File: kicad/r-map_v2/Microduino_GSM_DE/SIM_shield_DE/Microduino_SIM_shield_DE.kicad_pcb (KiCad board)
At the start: 2 copper layers, 25.5 x 27.9 mm, 15 parts, among them P1 CONN_1x27, P2 CONN_01X06, U1 TLV62569, U2 ESDA6V1-5W6

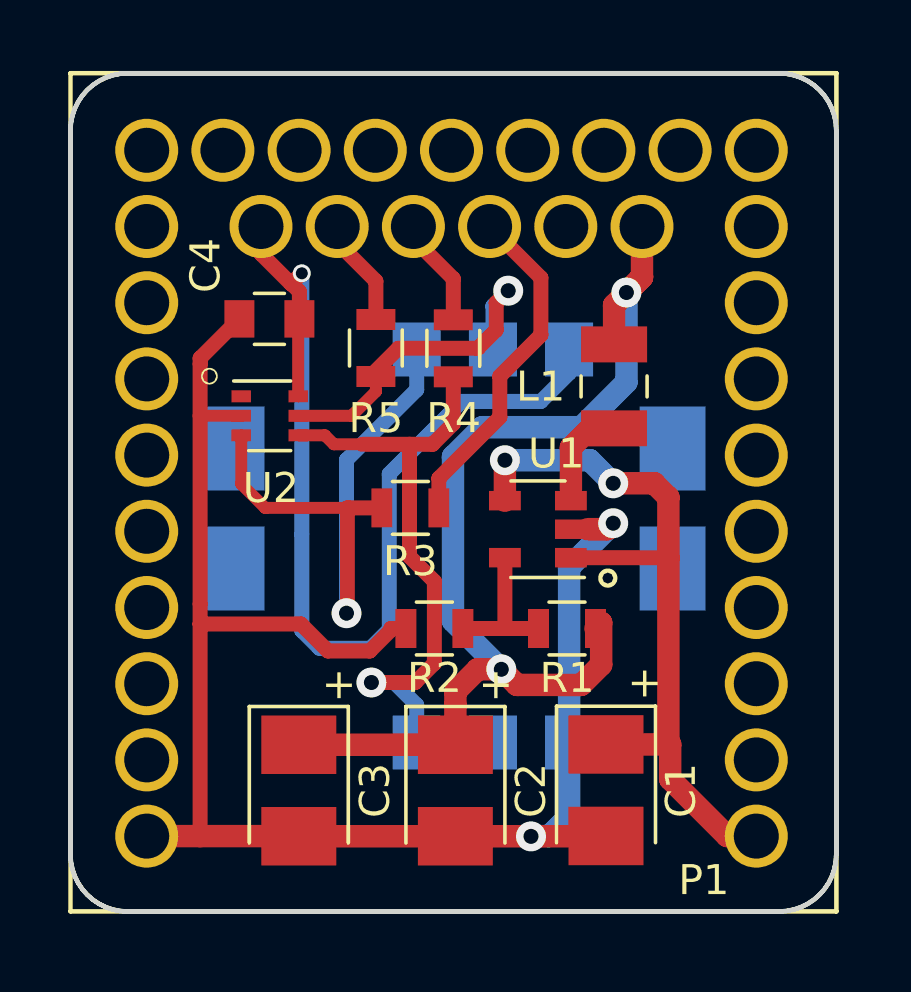
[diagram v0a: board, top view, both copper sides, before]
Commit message: kicad schemas update
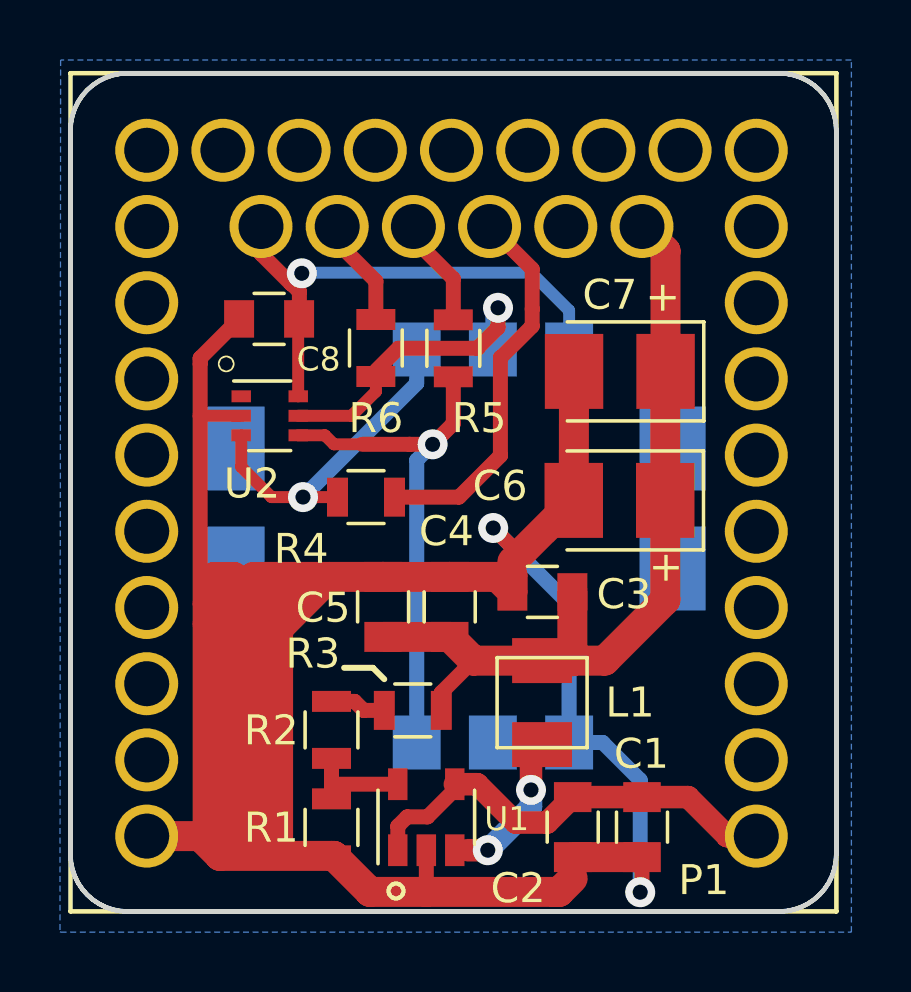
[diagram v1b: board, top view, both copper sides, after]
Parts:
- added C5: 100nF, Capacitors_SMD:C_0805, F.Cu at (149.1, 80.5)
- added C6: 100uF, Capacitors_Tantalum_SMD:CP_Tantalum_Case-B_EIA-3528-21_Reflow, F.Cu at (157.0, 77.0)
- added C7: 100uF, Capacitors_Tantalum_SMD:CP_Tantalum_Case-B_EIA-3528-21_Reflow, F.Cu at (157.0, 72.7)
- added C8: 100nF, Capacitors_SMD:C_0805, F.Cu at (145.3, 70.9)
- added R3: 560k, Resistors_SMD:R_0805, F.Cu at (150.1, 84.0)
- C1: value 100uF -> 4,7uF; footprint Capacitors_Tantalum_SMD:CP_Tantalum_Case-B_EIA-3528-21_Reflow -> Capacitors_SMD:C_0805
- C2: value 100uF -> 100nF; footprint Capacitors_Tantalum_SMD:CP_Tantalum_Case-B_EIA-3528-21_Reflow -> Capacitors_SMD:C_0805
- C3: value 100uF -> 10uF; footprint Capacitors_Tantalum_SMD:CP_Tantalum_Case-B_EIA-3528-21_Reflow -> Capacitors_SMD:C_0805
- C4: value 100nF -> 10uF
- L1: value 2,2 uH -> 1 uH; footprint Libreria_PCB_mia:Induttanza_SMD_2520_Wurth -> Libreria_PCB_mia:Induttanza_SMD_3030_Vishay
- R1: renamed from R2; value 56k -> 100k
- R2: renamed from R1; value 330k -> 10k
- R4: renamed from R3; value 22 -> 56
- R5: renamed from R4; value 22 -> 56
- R6: renamed from R5; value 22 -> 56
- moved C4 11.3 mm to (151.4, 80.5), turned to 90 degrees
- moved L1 10.8 mm to (154.4, 83.7)
- moved C3 10.5 mm to (154.4, 80.0), turned to 180 degrees
- moved U1 10.3 mm to (150.6, 87.5), turned to 90 degrees
- moved R2 8.55 mm to (147.4, 84.6), turned to 270 degrees
- moved R1 7.46 mm to (147.4, 87.9), turned to 270 degrees
- moved C2 4.10 mm to (155.5, 87.9)
- moved C1 1.72 mm to (157.8, 87.9)
- moved R4 1.52 mm to (148.6, 76.9)
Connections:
- net /VRTC renamed Net-(P2-Pad2)
- C2 pad 1: /VBAT -> +5V
- C4 pad 1: /VSIM -> /VBAT
- R2 pad 1: /VBAT -> Net-(R2-Pad1)
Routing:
- net GND: track 55.5 -> 134.4 mm
- net /VSIM: track 35.4 -> 17.5 mm
- net +5V: track 25.8 -> 16.8 mm, vias 2 -> 0
- net /SIM_CLK: track 20.0 -> 11.2 mm
- net /VBAT: track 36.9 -> 28.3 mm, vias 2 -> 0
- net /SIM_DATA: track 20.2 -> 17.3 mm
- net Net-(L1-Pad1): track 3.48 -> 5.57 mm, vias 0 -> 2
- net Net-(R2-Pad1): track 0.00 -> 1.88 mm
- net Net-(R1-Pad1): track 4.88 -> 3.56 mm
- net /SIM_RST: track 11.6 -> 10.5 mm
- net Net-(P2-Pad3): track 11.7 -> 12.8 mm
- added copper zone on B.Cu, net GND
